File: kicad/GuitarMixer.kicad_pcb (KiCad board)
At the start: 2 copper layers, 72.8 x 40.8 mm, 41 parts, among them J1 Conn_01x03_Pin, J2 Conn_01x03_Pin, J3 Conn_01x03_Pin, J4 Conn_01x02_Pin, J5 Conn_01x02_Pin, J6 Conn_01x03_Pin, Q1 2N5457, SW1 SW_SPST, U1 TL072, U2 TL072

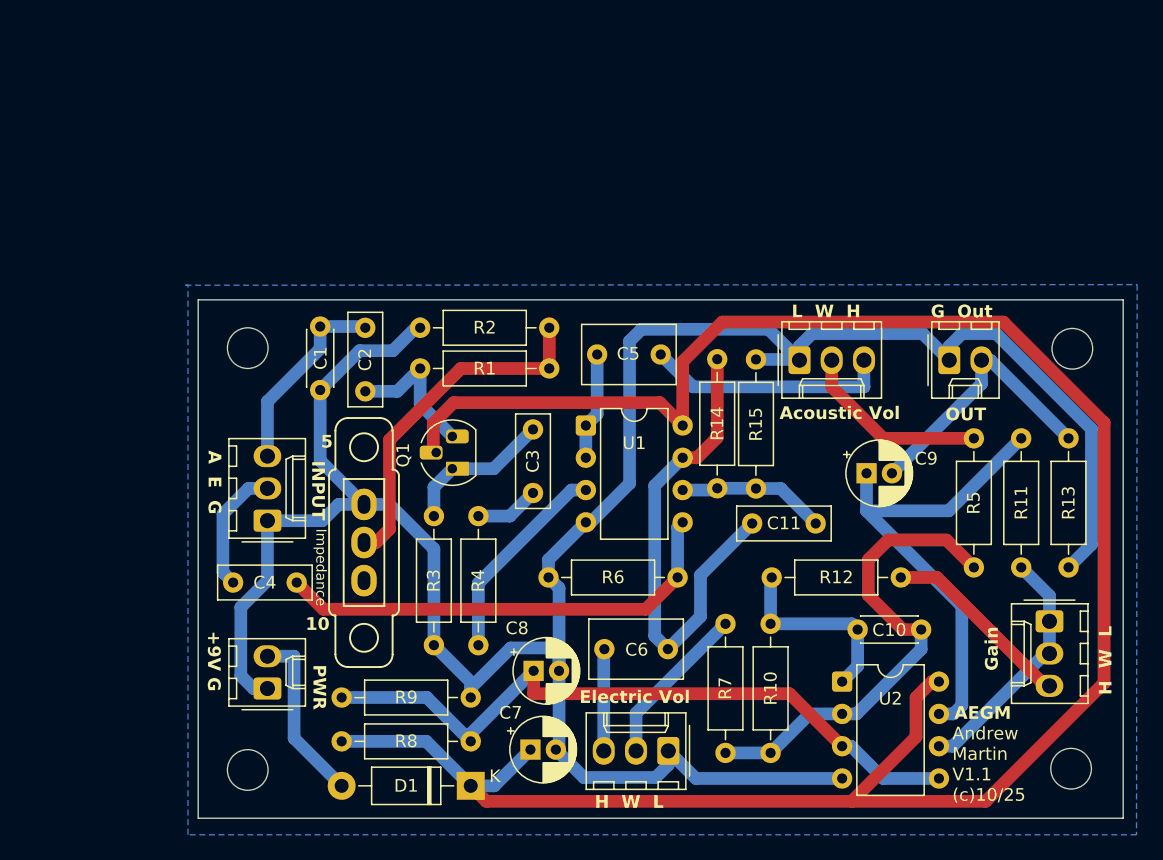
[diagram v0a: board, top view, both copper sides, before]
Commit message: Board created
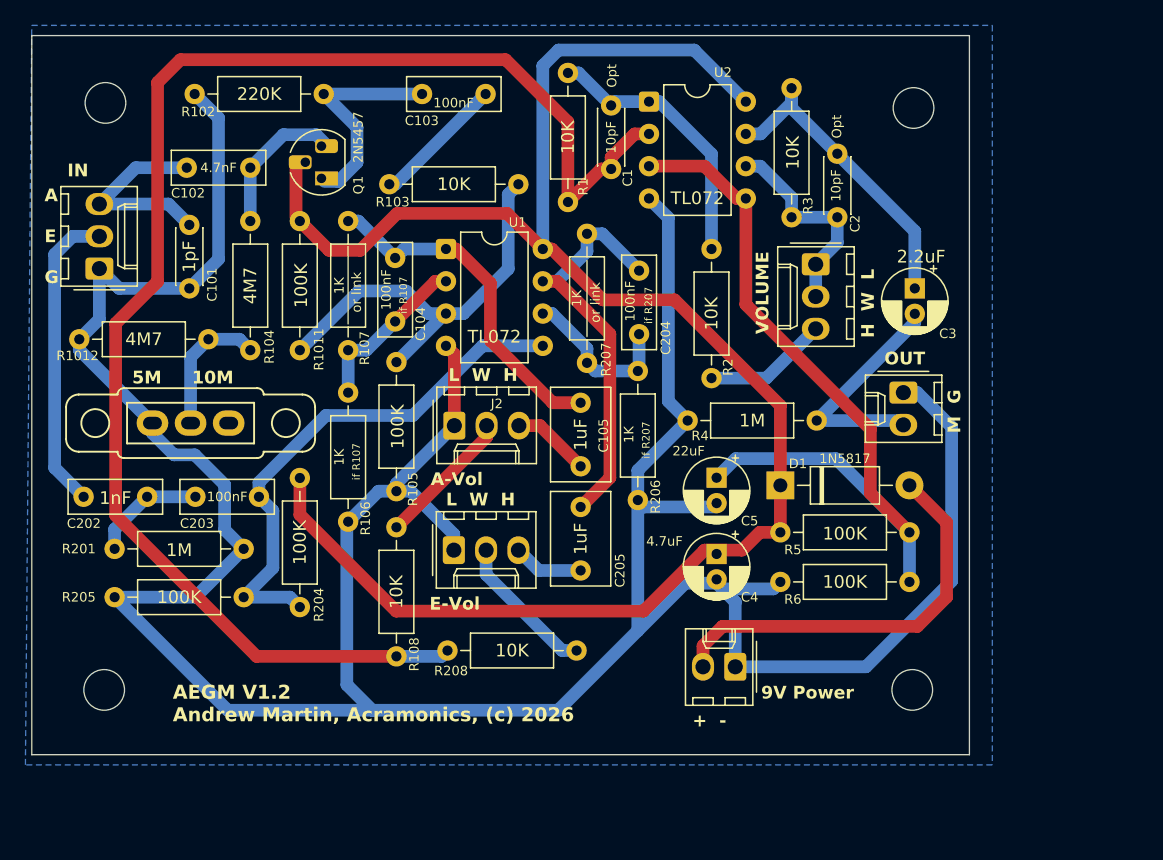
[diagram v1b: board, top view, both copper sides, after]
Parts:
- removed C10: 10pF, Capacitor_THT:C_Disc_D4.3mm_W1.9mm_P5.00mm
- removed C11: 100nF, Capacitor_THT:C_Rect_L7.2mm_W2.5mm_P5.00mm_FKS2_FKP2_MKS2_MKP2
- removed C6: 1uF, Capacitor_THT:C_Rect_L7.2mm_W4.5mm_P5.00mm_FKS2_FKP2_MKS2_MKP2
- removed C7: 4.7uF, Capacitor_THT:CP_Radial_D5.0mm_P2.00mm
- removed C8: 22uF, Capacitor_THT:CP_Radial_D5.0mm_P2.00mm
- removed C9: 2.2uF, Capacitor_THT:CP_Radial_D5.0mm_P2.00mm
- removed R10, R12, R7: 10K, Resistor_THT:R_Axial_DIN0207_L6.3mm_D2.5mm_P10.16mm_Horizontal
- removed R11, R8, R9: 100K, Resistor_THT:R_Axial_DIN0207_L6.3mm_D2.5mm_P10.16mm_Horizontal
- removed R13: 1M, Resistor_THT:R_Axial_DIN0207_L6.3mm_D2.5mm_P10.16mm_Horizontal
- removed R14, R15: 1K, Resistor_THT:R_Axial_DIN0207_L6.3mm_D2.5mm_P10.16mm_Horizontal
- removed the REF** at (183.9, 79.0)
- removed the REF** at (119.0, 112.2)
- removed the REF** at (183.8, 112.1)
- removed the REF** at (119.0, 79.0)
- added C101: 1pF, Capacitor_THT:C_Disc_D4.3mm_W1.9mm_P5.00mm, F.Cu at (114.4, 69.3)
- added C102: 4.7nF, Capacitor_THT:C_Rect_L7.2mm_W2.5mm_P5.00mm_FKS2_FKP2_MKS2_MKP2, F.Cu at (114.2, 64.8)
- added C103: 100nF, Capacitor_THT:C_Rect_L7.2mm_W2.5mm_P5.00mm_FKS2_FKP2_MKS2_MKP2, F.Cu at (132.7, 59.0)
- added C104: 100nF, Capacitor_THT:C_Rect_L7.2mm_W2.5mm_P5.00mm_FKS2_FKP2_MKS2_MKP2, F.Cu at (130.6, 76.9)
- added C105: 1uF, Capacitor_THT:C_Rect_L7.2mm_W4.5mm_P5.00mm_FKS2_FKP2_MKS2_MKP2, F.Cu at (145.2, 83.3)
- added C202: 1nF, Capacitor_THT:C_Rect_L7.2mm_W2.5mm_P5.00mm_FKS2_FKP2_MKS2_MKP2, F.Cu at (106.1, 90.7)
- added C203: 100nF, Capacitor_THT:C_Rect_L7.2mm_W2.5mm_P5.00mm_FKS2_FKP2_MKS2_MKP2, F.Cu at (114.9, 90.7)
- added C204: 100nF, Capacitor_THT:C_Rect_L7.2mm_W2.5mm_P5.00mm_FKS2_FKP2_MKS2_MKP2, F.Cu at (149.8, 77.9)
- added C205: 1uF, Capacitor_THT:C_Rect_L7.2mm_W4.5mm_P5.00mm_FKS2_FKP2_MKS2_MKP2, F.Cu at (145.2, 91.5)
- added R1011: 4M7, Resistor_THT:R_Axial_DIN0207_L6.3mm_D2.5mm_P10.16mm_Horizontal, F.Cu at (119.2, 69.0)
- added R1012: 4M7, Resistor_THT:R_Axial_DIN0207_L6.3mm_D2.5mm_P10.16mm_Horizontal, F.Cu at (115.9, 78.3)
- added R102: 220K, Resistor_THT:R_Axial_DIN0207_L6.3mm_D2.5mm_P10.16mm_Horizontal, F.Cu at (125.0, 59.0)
- added R103: 10K, Resistor_THT:R_Axial_DIN0207_L6.3mm_D2.5mm_P10.16mm_Horizontal, F.Cu at (130.1, 66.1)
- added R104: 100K, Resistor_THT:R_Axial_DIN0207_L6.3mm_D2.5mm_P10.16mm_Horizontal, F.Cu at (123.1, 79.2)
- added R105: 100K, Resistor_THT:R_Axial_DIN0207_L6.3mm_D2.5mm_P10.16mm_Horizontal, F.Cu at (130.7, 90.3)
- added R106: 1K, Resistor_THT:R_Axial_DIN0207_L6.3mm_D2.5mm_P10.16mm_Horizontal, F.Cu at (126.9, 82.5)
- added R107: 1K, Resistor_THT:R_Axial_DIN0207_L6.3mm_D2.5mm_P10.16mm_Horizontal, F.Cu at (126.9, 79.2)
- added R108: 10K, Resistor_THT:R_Axial_DIN0207_L6.3mm_D2.5mm_P10.16mm_Horizontal, F.Cu at (130.7, 93.1)
- added R201: 1M, Resistor_THT:R_Axial_DIN0207_L6.3mm_D2.5mm_P10.16mm_Horizontal, F.Cu at (108.5, 94.8)
- added R204: 100K, Resistor_THT:R_Axial_DIN0207_L6.3mm_D2.5mm_P10.16mm_Horizontal, F.Cu at (123.1, 99.4)
- added R205: 100K, Resistor_THT:R_Axial_DIN0207_L6.3mm_D2.5mm_P10.16mm_Horizontal, F.Cu at (108.5, 98.6)
- added R206: 1K, Resistor_THT:R_Axial_DIN0207_L6.3mm_D2.5mm_P10.16mm_Horizontal, F.Cu at (149.7, 80.8)
- added R207: 1K, Resistor_THT:R_Axial_DIN0207_L6.3mm_D2.5mm_P10.16mm_Horizontal, F.Cu at (145.7, 80.2)
- added R208: 10K, Resistor_THT:R_Axial_DIN0207_L6.3mm_D2.5mm_P10.16mm_Horizontal, F.Cu at (144.9, 102.8)
- added REF**: MountingHole_3.2mm_M3, MountingHole:MountingHole_3.2mm_M3, F.Cu at (107.8, 59.7)
- added REF**: MountingHole_3.2mm_M3, MountingHole:MountingHole_3.2mm_M3, F.Cu at (171.3, 105.9)
- added REF**: MountingHole_3.2mm_M3, MountingHole:MountingHole_3.2mm_M3, F.Cu at (171.4, 60.1)
- added REF**: MountingHole_3.2mm_M3, MountingHole:MountingHole_3.2mm_M3, F.Cu at (107.7, 105.9)
- C1: value 1pF -> 10pF
- C2: value 33nF -> 10pF; footprint Capacitor_THT:C_Rect_L7.2mm_W2.5mm_P5.00mm_FKS2_FKP2_MKS2_MKP2 -> Capacitor_THT:C_Disc_D4.3mm_W1.9mm_P5.00mm
- C3: value 100nF -> 2.2uF; footprint Capacitor_THT:C_Rect_L7.2mm_W2.5mm_P5.00mm_FKS2_FKP2_MKS2_MKP2 -> Capacitor_THT:CP_Radial_D5.0mm_P2.00mm
- C4: value 100nF -> 4.7uF; footprint Capacitor_THT:C_Rect_L7.2mm_W2.5mm_P5.00mm_FKS2_FKP2_MKS2_MKP2 -> Capacitor_THT:CP_Radial_D5.0mm_P2.00mm
- C5: value 1uF -> 22uF; footprint Capacitor_THT:C_Rect_L7.2mm_W4.5mm_P5.00mm_FKS2_FKP2_MKS2_MKP2 -> Capacitor_THT:CP_Radial_D5.0mm_P2.00mm
- R1, R2: value 4M7 -> 10K
- R3: value 220K -> 10K
- R4: value 10K -> 1M
- R5: value 10K -> 100K
- R6: value 1M -> 100K
- moved U2 48.1 mm to (150.6, 59.6)
- moved C2 38.2 mm to (165.4, 68.7), turned to 90 degrees
- moved C4 38.1 mm to (155.9, 95.2), turned to -90 degrees
- moved J4 36.9 mm to (157.4, 104.1), turned to 180 degrees
- moved R3 36.7 mm to (161.8, 68.7), turned to 90 degrees
- moved D1 34.0 mm to (160.9, 89.8), turned to 0 degrees
- moved J6 33.6 mm to (163.7, 72.4)
- moved C3 32.0 mm to (171.5, 74.3)
- moved J2 27.6 mm to (135.3, 85.1)
- moved C1 26.0 mm to (147.6, 64.9), turned to 90 degrees
- moved Q1 25.1 mm to (124.8, 65.6)
- moved J1 23.8 mm to (107.3, 72.7)
- moved J3 23.1 mm to (135.2, 94.9), turned to 0 degrees
- moved R4 18.1 mm to (153.6, 84.7), turned to 0 degrees
- moved U1 17.7 mm to (134.6, 71.2)
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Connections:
- C1 pad 1: Net-(J1-Pin_3) -> Net-(U2A--)
- C1 pad 2: Earth -> Net-(C1-Pad2)
- C2 pad 1: Net-(J1-Pin_3) -> Net-(J6-Pin_1)
- C2 pad 2: Net-(Q1-G) -> Net-(C2-Pad2)
- C3 pad 1: Net-(Q1-S) -> Net-(C2-Pad2)
- C3 pad 2: Net-(C3-Pad2) -> Net-(J5-Pin_2)
- C4 pad 1: Net-(J1-Pin_2) -> +9VA
- C4 pad 2: Net-(U1B-+) -> Earth
- C5 pad 1: Net-(U1A--) -> +4V
- C5 pad 2: Net-(J2-Pin_3) -> Earth
- R1 pad 1: Net-(Q1-G) -> Net-(U2A--)
- R1 pad 2: Net-(SW1-B) -> Net-(C1-Pad2)
- R2 pad 1: Net-(SW1-B) -> Net-(J6-Pin_3)
- R2 pad 2: Earth -> Net-(C1-Pad2)
- R3 pad 1: Net-(Q1-S) -> Net-(J6-Pin_1)
- R3 pad 2: Earth -> Net-(C2-Pad2)
- R4 pad 1: Net-(C3-Pad2) -> Earth
- R4 pad 2: Net-(U1A-+) -> Net-(J5-Pin_2)
- R5 pad 1: Net-(J2-Pin_2) -> +4V
- R5 pad 2: Net-(U2A--) -> +9VA
- R6 pad 1: Net-(U1B-+) -> Earth
- R6 pad 2: Earth -> +4V
- U1 pad 1: Net-(U1A--) -> Net-(C104-Pad2)
- U2 pad 1: Net-(C10-Pad2) -> Net-(C1-Pad2)
- U2 pad 7: Net-(C9-Pad1) -> Net-(C2-Pad2)
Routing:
- net Net-(U2A--): track 38.2 -> 116.8 mm
- net Earth: track 195.7 -> 253.8 mm
- net Net-(C9-Pad1): track 38.0 -> 0.00 mm
- net +9VA: track 171.0 -> 140.0 mm
- net Net-(C104-Pad2): track 0.00 -> 27.4 mm
- net Net-(C2-Pad2): track 0.00 -> 25.2 mm
- net Net-(C1-Pad2): track 0.00 -> 21.7 mm
- net +9V: track 13.8 -> 32.4 mm
- net Net-(SW1-B): track 27.9 -> 10.8 mm
- net Net-(U1A-+): track 16.4 -> 33.0 mm
- net Net-(C10-Pad2): track 15.3 -> 0.00 mm
- net Net-(J1-Pin_2): track 10.1 -> 24.1 mm
- net Net-(J2-Pin_3): track 19.2 -> 6.19 mm
- net Net-(C103-Pad2): track 0.00 -> 10.5 mm
- net Net-(C202-Pad2): track 0.00 -> 8.96 mm
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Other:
- board size 72.8 x 40.8 mm -> 73.8 x 56.6 mm
- board text added: "+ -"
- board text added: "5M 10M"
- board text added: "9V Power"
- board text added: "A-Vol"
- board text added: "AEGM V1.2 Andrew Martin, Acramonics, (c) 2026"
- board text added: "E-Vol"
- board text added: "IN"
- board text added: "M G"
- board text added: "Opt"
- board text added: "VOLUME"
- board text added: "if R107"
- board text added: "if R207"
- board text added: "or link"
- board text removed: "+9V G"
- board text removed: "10"
- board text removed: "5"
- board text removed: "AEGM"
- board text removed: "Acoustic Vol"
- board text removed: "Andrew Martin V1.1 (c)10/25"
- board text removed: "Electric Vol"
- board text removed: "G Out"
- board text removed: "Gain"
- board text removed: "INPUT"
- board text removed: "Impedance"
- board text removed: "PWR"
